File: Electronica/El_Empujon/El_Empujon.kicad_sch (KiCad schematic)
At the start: 0 parts

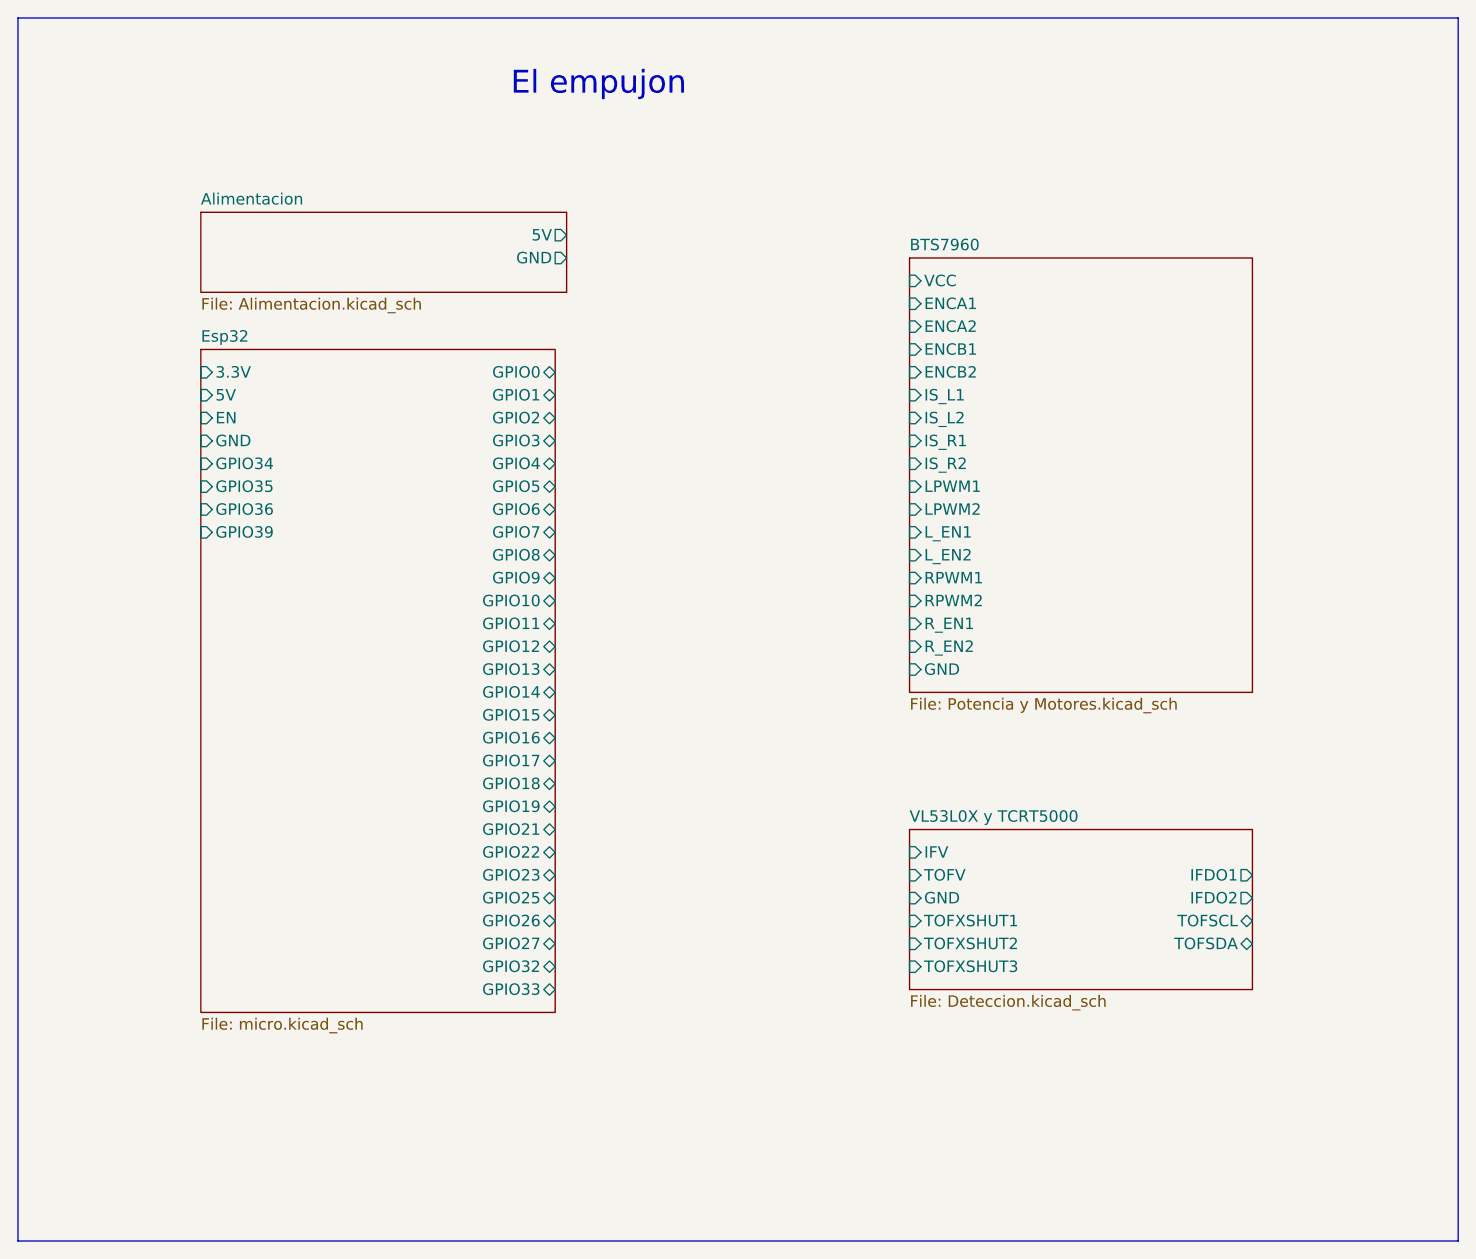
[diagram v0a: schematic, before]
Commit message: Generacion del STEP, finalizacion del esquematico y de la PCB, generacion de los archivos de manufactura de la PCB, Pedido de la PCB y actualizacion del Presupuesto.
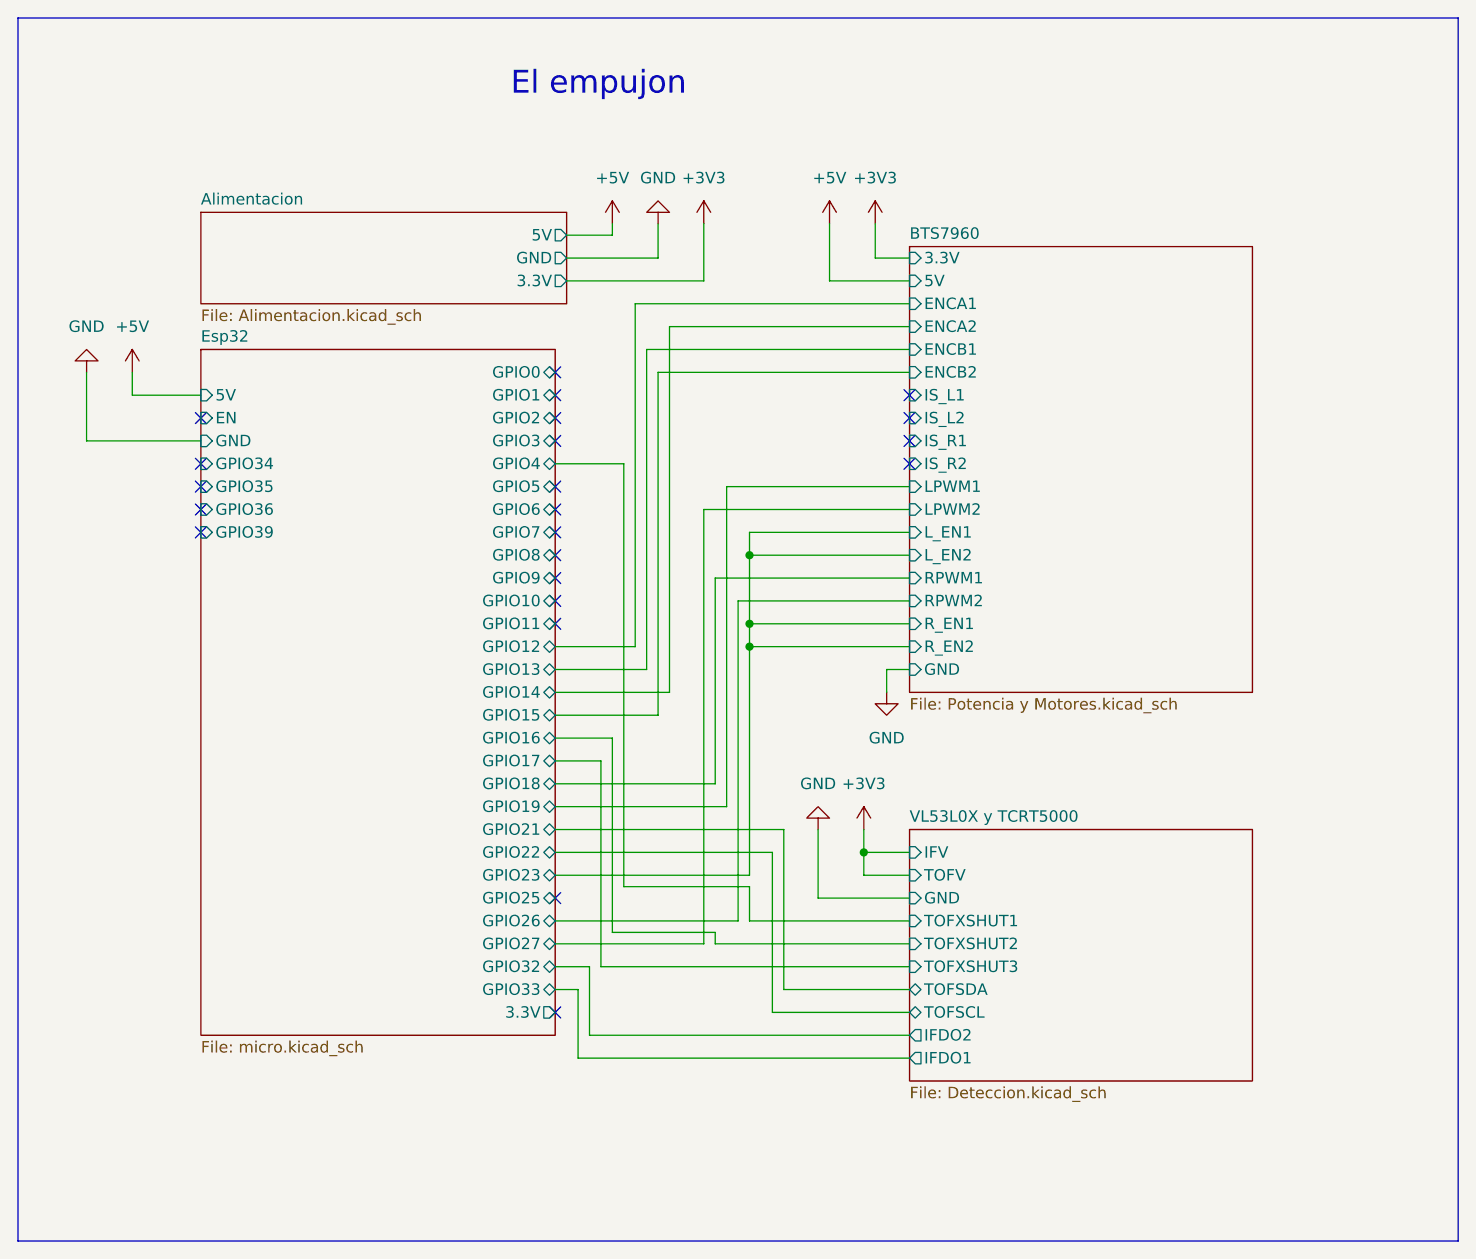
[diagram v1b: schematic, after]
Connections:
- no-connect marks 0 -> 22
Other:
- sheet Alimentacion ports: added 3.3V; removed none
- sheet BTS7960 ports: added 3.3V, 5V; removed VCC
